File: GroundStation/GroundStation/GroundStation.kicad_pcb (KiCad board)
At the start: 2 copper layers, 70 parts, among them J1 SD_Card_Receptacle, J4 Conn_Coaxial, J5 Conn_01x02, P1 USB_C_Plug_USB2.0, Q1 TSM3481CX6 RFG, U1 STM32F103C8Tx, U101 LD1117S33TR_SOT223, U2 E22-400T30S_LoRa, U4 TPS54538RQFR, U9 NEO-M9N-00B

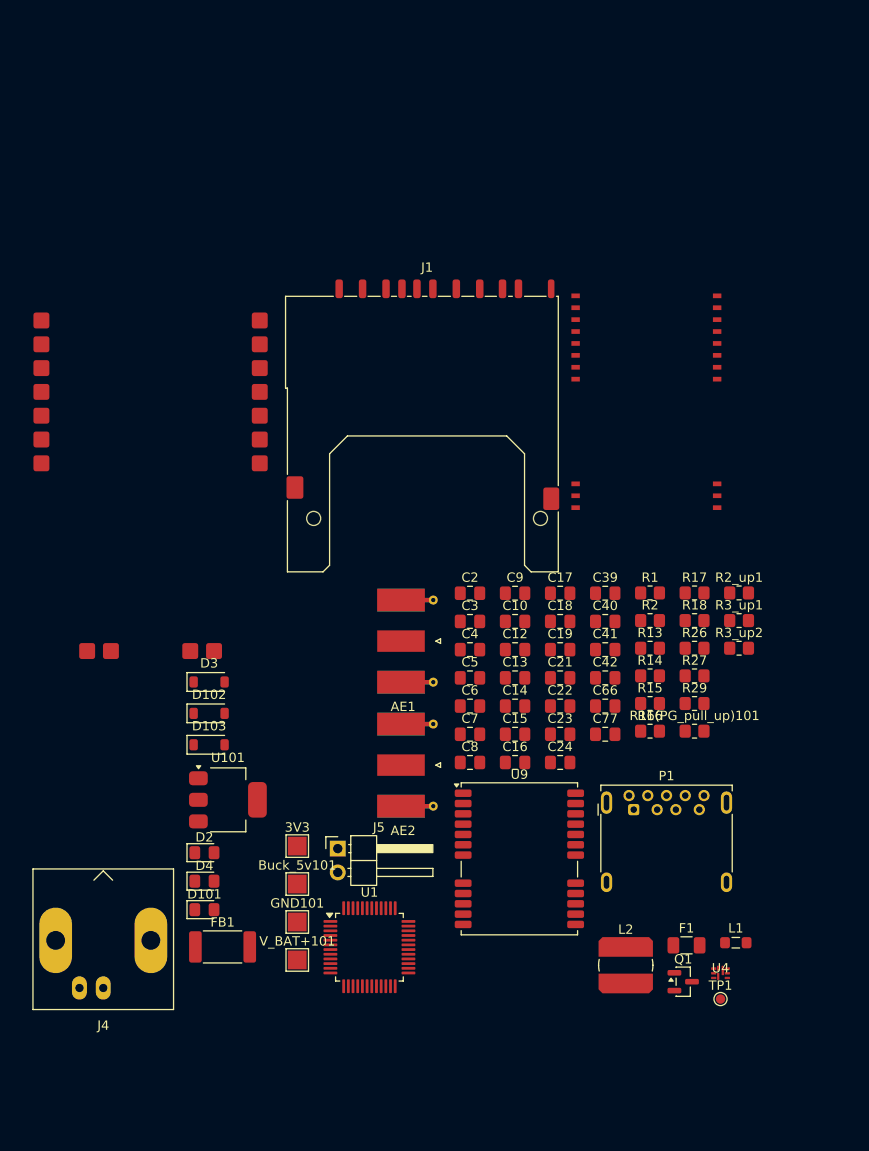
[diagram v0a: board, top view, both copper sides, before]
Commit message: Ray Wanted to try free routing
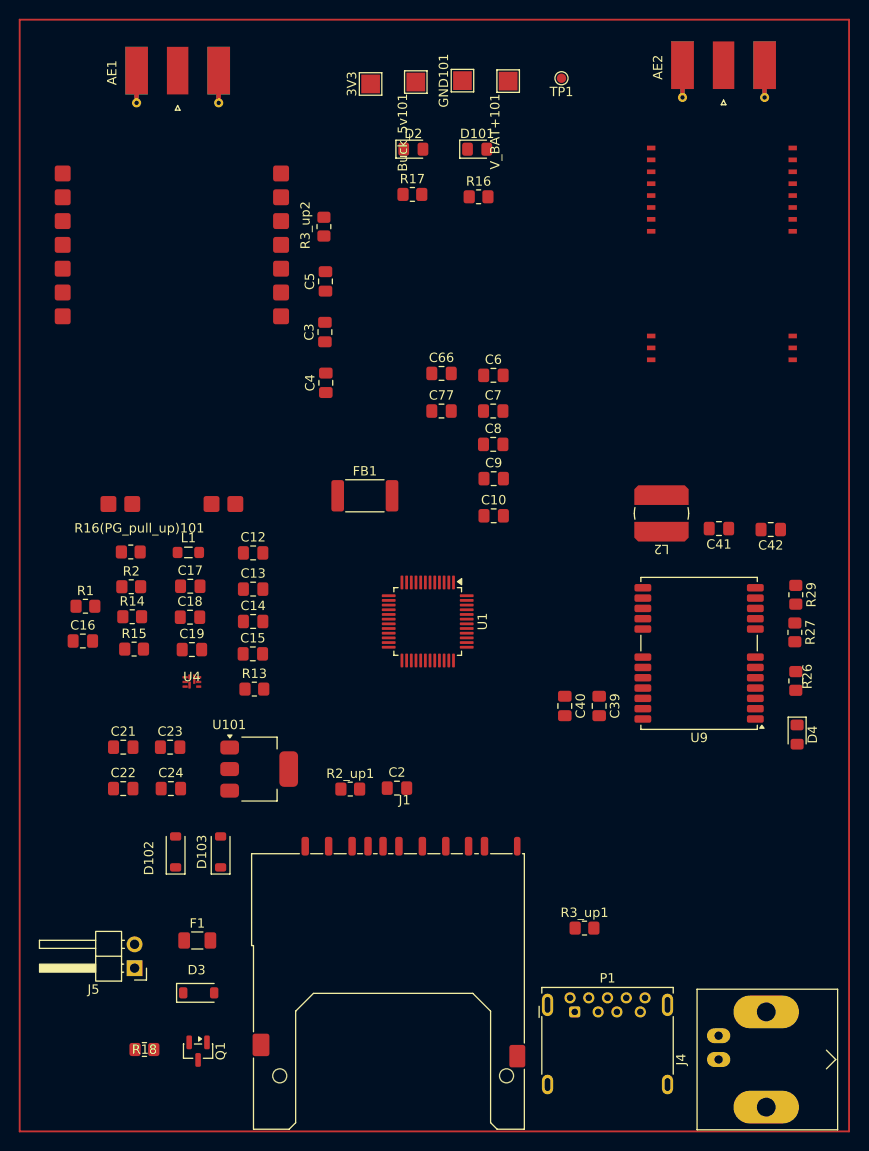
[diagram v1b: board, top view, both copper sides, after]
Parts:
- moved TP1 99.7 mm to (146.6, 29.3), turned to 180 degrees
- moved V_BAT+101 96.4 mm to (140.9, 29.6), turned to 90 degrees
- moved GND101 91.5 mm to (136.0, 29.6), turned to 90 degrees
- moved Buck_5v101 86.5 mm to (131.1, 29.7), turned to 90 degrees
- moved D101 86.2 mm to (137.6, 36.9)
- moved 3V3 81.7 mm to (126.2, 29.9), turned to 90 degrees
- moved AE2 79.9 mm to (163.9, 29.6), turned to -90 degrees
- moved D2 78.3 mm to (130.8, 36.9)
- moved R18 74.4 mm to (102.1, 132.9)
- moved L1 71.7 mm to (106.8, 79.9)
- moved J4 66.1 mm to (163.4, 134.0), turned to -90 degrees
- moved D4 65.1 mm to (171.7, 99.3), turned to -90 degrees
- moved AE1 64.4 mm to (105.7, 30.2), turned to -90 degrees
- moved U4 64.4 mm to (107.2, 93.7)
- moved R3_up2 63.1 mm to (121.3, 45.1), turned to 90 degrees
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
